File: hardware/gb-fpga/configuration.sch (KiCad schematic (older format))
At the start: 13 parts, among them U1 xc7s25ftgb196, U2 MX25R3235FZBxx1

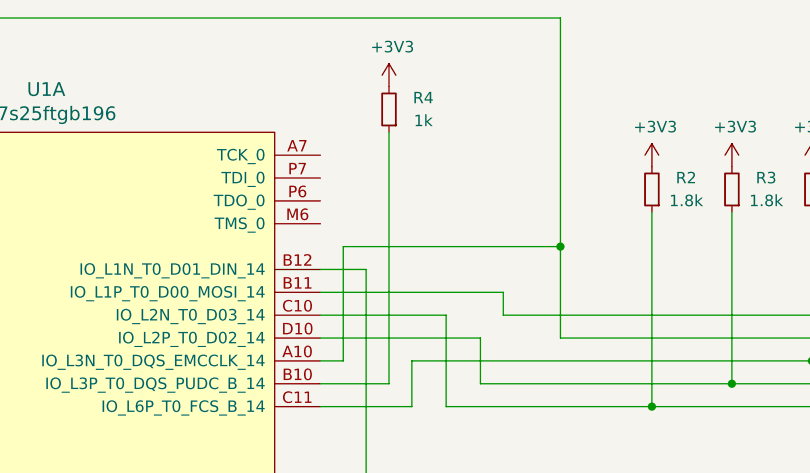
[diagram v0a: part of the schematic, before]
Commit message: Add USB connections
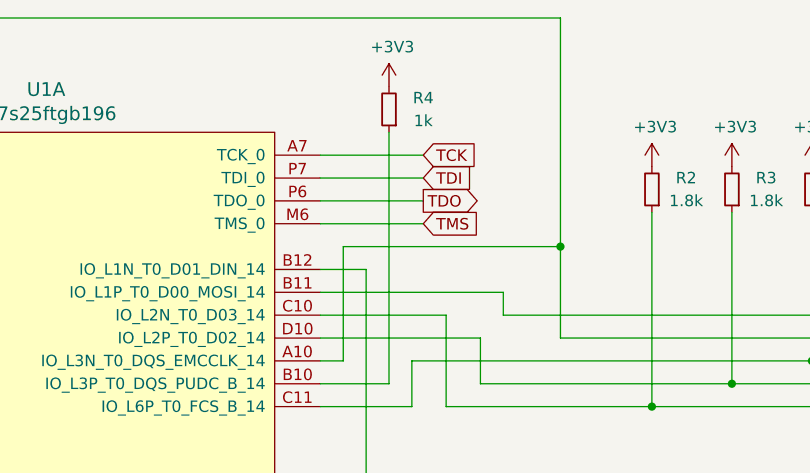
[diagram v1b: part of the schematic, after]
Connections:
- net TCK: now reaches U1.A7 (TCK_0)
- net TMS: now reaches U1.M6 (TMS_0)
- net TDO: now reaches U1.P6 (TDO_0)
- net TDI: now reaches U1.P7 (TDI_0)
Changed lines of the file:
@@
 	5400 4300 5700 4300
-Wire Wire Line
-	5700 4300 5700 3200
-$Comp
-L Device:R_Small R4
-U 1 1 60DA54B4
-P 5700 3100
-F 0 "R4" H 5550 3050 50  0000 C CNN
-F 1 "1k" H 5550 3150 50  0000 C CNN
-F 2 "Resistor_SMD:R_0603_1608Metric" H 5700 3100 50  0001 C CNN
-F 3 "~" H 5700 3100 50  0001 C CNN
-	1    5700 3100
-	-1   0    0    1
-$EndComp
-$Comp
-L power:+3V3 #PWR0111
-U 1 1 60DA5CD7
-P 5700 3000
-F 0 "#PWR0111" H 5700 2850 50  0001 C CNN
-F 1 "+3V3" H 5715 3173 50  0000 C CNN
-F 2 "" H 5700 3000 50  0001 C CNN
-F 3 "" H 5700 3000 50  0001 C CNN
-	1    5700 3000
-	1    0    0    -1
-$EndComp
 Wire Wire Line
 	3000 3400 2300 3400
@@
 Wire Wire Line
 	2150 5100 2150 4900
+$Comp
+L power:+3V3 #PWR0111
+U 1 1 60DA5CD7
+P 5700 3000
+F 0 "#PWR0111" H 5700 2850 50  0001 C CNN
+F 1 "+3V3" H 5715 3173 50  0000 C CNN
+F 2 "" H 5700 3000 50  0001 C CNN
+F 3 "" H 5700 3000 50  0001 C CNN
+	1    5700 3000
+	1    0    0    -1
+$EndComp
+Wire Wire Line
+	5700 4300 5700 3200
+$Comp
+L Device:R_Small R4
+U 1 1 60DA54B4
+P 5700 3100
+F 0 "R4" H 5550 3050 50  0000 C CNN
+F 1 "1k" H 5550 3150 50  0000 C CNN
+F 2 "Resistor_SMD:R_0603_1608Metric" H 5700 3100 50  0001 C CNN
+F 3 "~" H 5700 3100 50  0001 C CNN
+	1    5700 3100
+	-1   0    0    1
+$EndComp
+Wire Wire Line
+	5400 3300 5850 3300
+Wire Wire Line
+	5400 3400 5850 3400
+Wire Wire Line
+	5400 3500 5850 3500
+Wire Wire Line
+	5400 3600 5850 3600
+Text GLabel 5850 3300 2    50   Input ~ 0
+TCK
+Text GLabel 5850 3400 2    50   Input ~ 0
+TDI
+Text GLabel 5850 3500 2    50   Output ~ 0
+TDO
+Text GLabel 5850 3600 2    50   Input ~ 0
+TMS
 $EndSCHEMATC
